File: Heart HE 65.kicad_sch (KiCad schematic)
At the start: 61 parts, among them J6 Conn_01x04, SW1 SW_Push, U1 PRTR5V0U2X, U19 AP2112K-3.3, U27 AT32F405KxU7-4, U63 AMS1117-3.3, U85 TPS63001, Y1 12Mhz (15p)

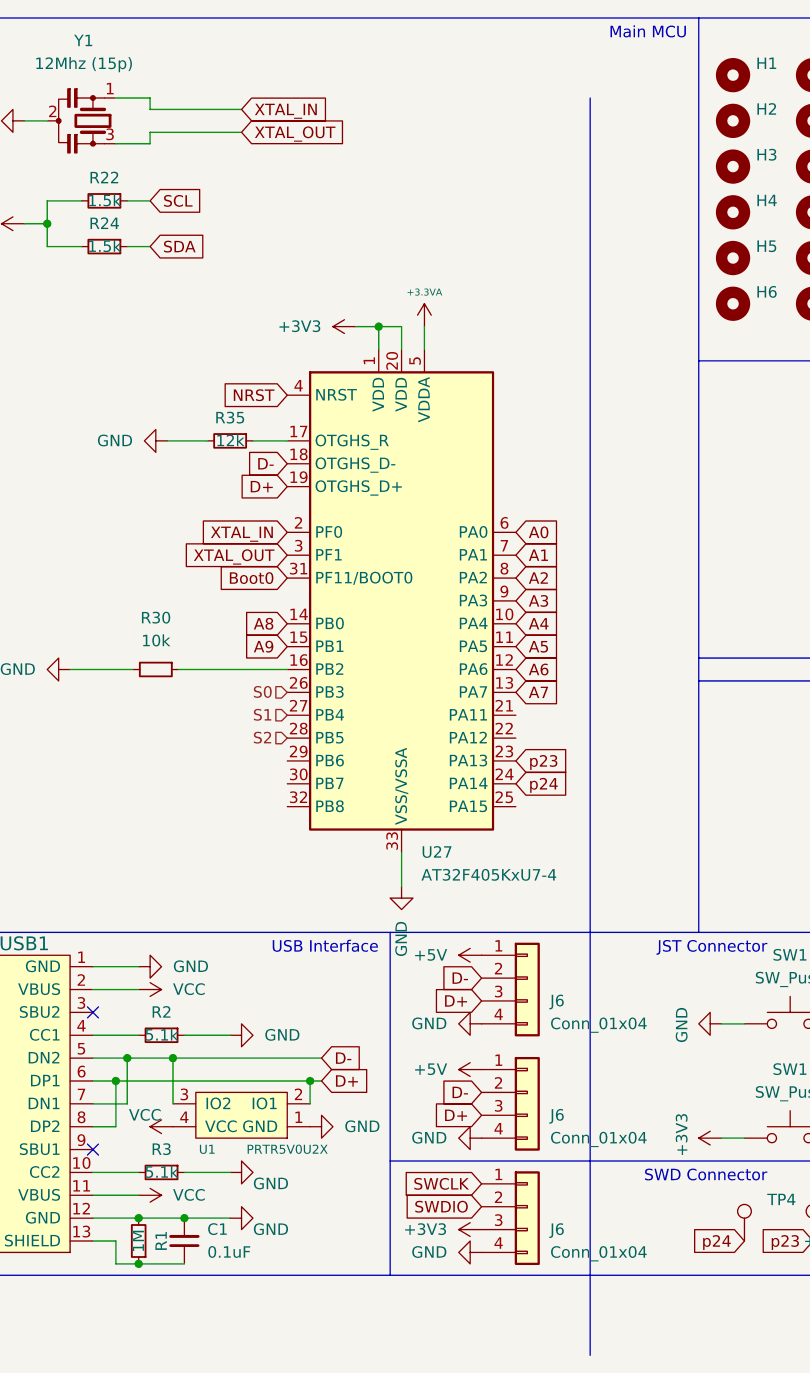
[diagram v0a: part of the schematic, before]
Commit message: Change
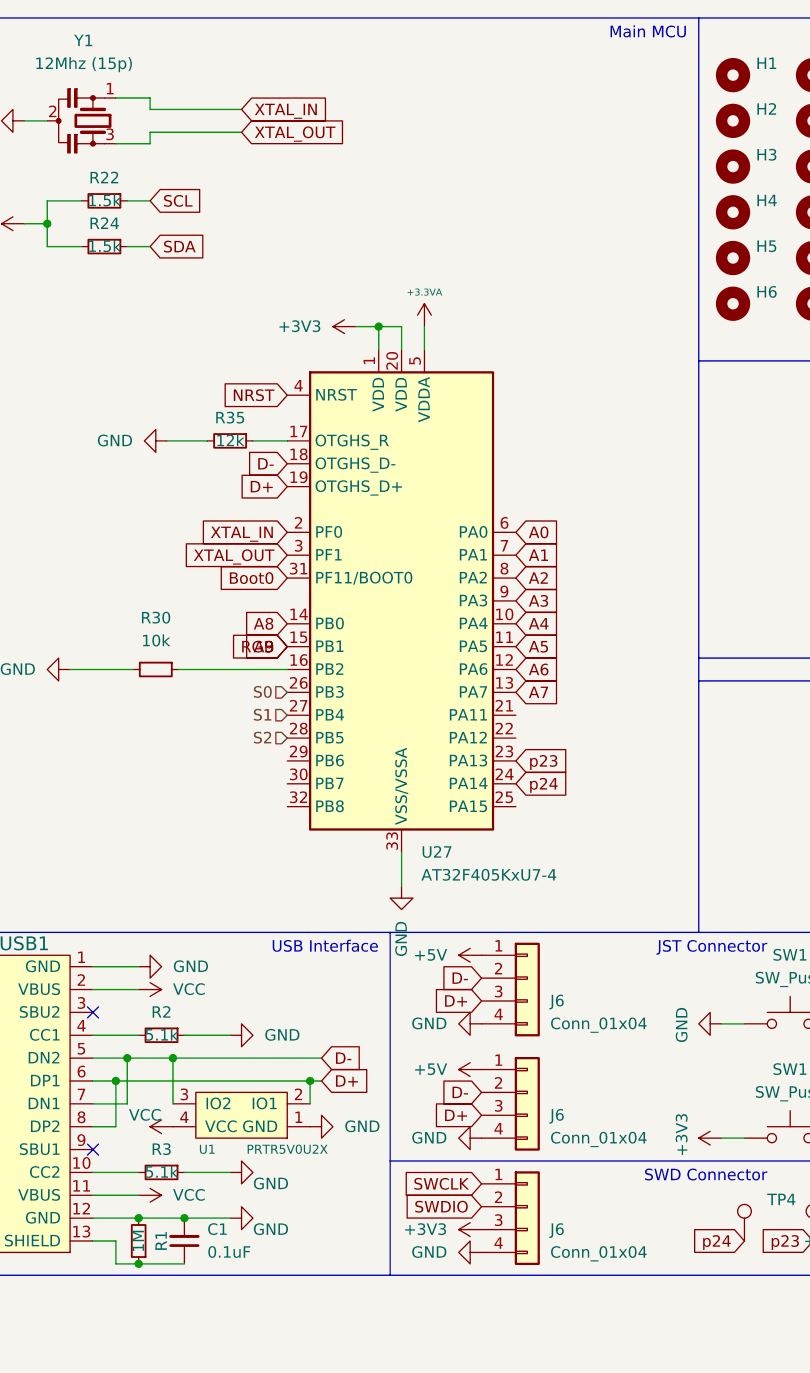
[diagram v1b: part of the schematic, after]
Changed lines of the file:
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@@
-		)
-	)
-	(polyline
-		(pts
-			(xy 85.725 66.04) (xy 85.725 205.74)
-		)
-		(stroke
-			(width 0)
-			(type default)
 		)
 	)
@@
 				(hide yes)
 			)
+		)
+	)
+	(global_label "RGB"
+		(shape input)
+		(at 52.07 127 180)
+		(fields_autoplaced yes)
+		(effects
+			(font
+				(size 1.27 1.27)
+			)
+			(justify right)
+		)
+		(property "Intersheetrefs" "${INTERSHEET_REFS}"
+			(at 45.2748 127 0)
+			(effects
+				(font
+					(size 1.27 1.27)
+				)
+				(justify right)
+				(hide yes)
+			)
